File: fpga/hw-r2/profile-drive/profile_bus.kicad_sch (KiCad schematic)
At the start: 13 parts, among them J2 NorComp 182-025-213R561, U1 LFE5U-12F-6TG144C, U2 74LVC245A DATA, U3 74LVC245A CTRL-IN

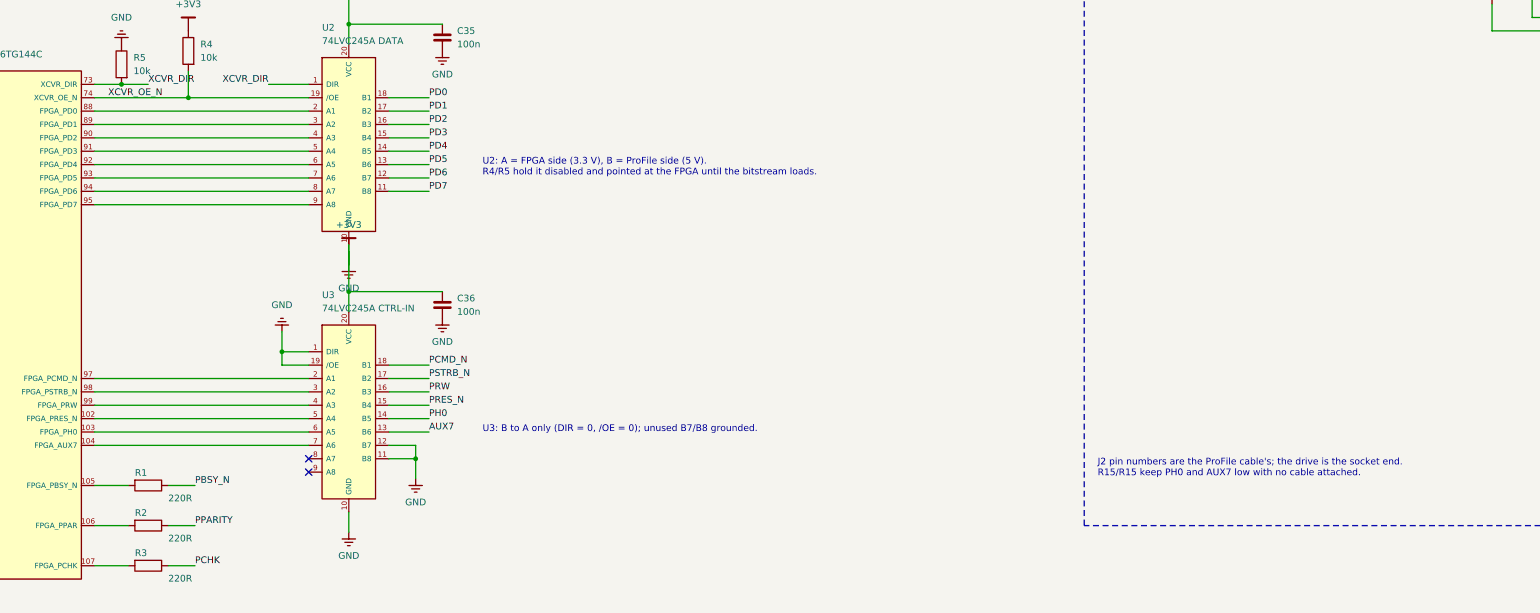
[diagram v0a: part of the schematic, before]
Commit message: more fixes, and r2 gerber first pass
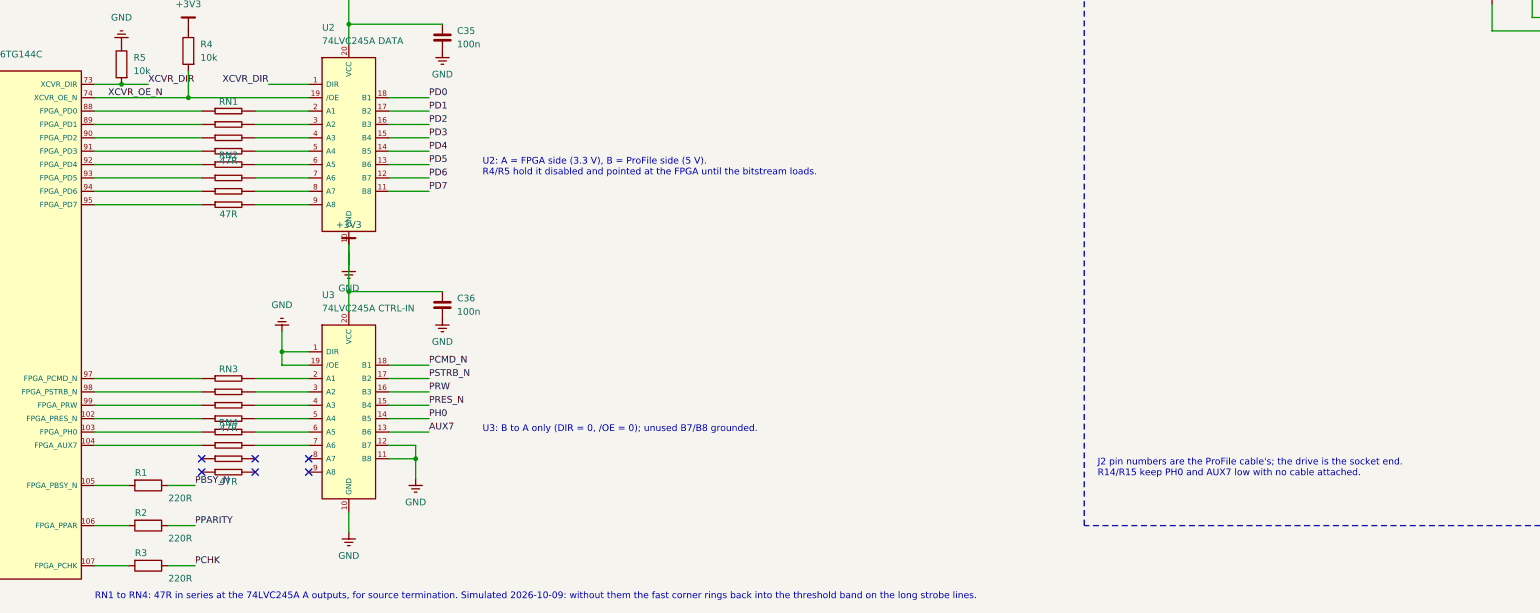
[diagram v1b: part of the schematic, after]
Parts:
- added RN1, RN2, RN3, RN4: 47R, Resistor_SMD:R_Array_Convex_4x0603, symbol device:R_Pack04
- C35, C36: MPN (none) -> Samsung CL10B104KO8NNNC
- J2: MPN (none) -> NorComp 182-025-213R561
- R1, R2, R3: MPN (none) -> Yageo RC0603FR-07220RL
- R14, R15: MPN (none) -> Yageo RC0603FR-07100KL
- R4, R5: MPN (none) -> Yageo RC0603FR-0710KL
- U1: MPN (none) -> Lattice LFE5U-12F-6TG144C
- U2, U3: MPN (none) -> TI SN74LVC245APWR
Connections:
- net at U1.102 (FPGA_PRES_N): now also RN3.4; no longer U3.5 (A4)
- net at U1.103 (FPGA_PH0): now also RN4.1; no longer U3.6 (A5)
- net at U1.104 (FPGA_AUX7): now also RN4.2; no longer U3.7 (A6)
- net at U1.88 (FPGA_PD0): now also RN1.1; no longer U2.2 (A1)
- net at U1.89 (FPGA_PD1): now also RN1.2; no longer U2.3 (A2)
- net at U1.90 (FPGA_PD2): now also RN1.3; no longer U2.4 (A3)
- net at U1.91 (FPGA_PD3): now also RN1.4; no longer U2.5 (A4)
- net at U1.92 (FPGA_PD4): now also RN2.1; no longer U2.6 (A5)
- net at U1.93 (FPGA_PD5): now also RN2.2; no longer U2.7 (A6)
- net at U1.94 (FPGA_PD6): now also RN2.3; no longer U2.8 (A7)
- net at U1.95 (FPGA_PD7): now also RN2.4; no longer U2.9 (A8)
- net at U1.97 (FPGA_PCMD_N): now also RN3.1; no longer U3.2 (A1)
- net at U1.98 (FPGA_PSTRB_N): now also RN3.2; no longer U3.3 (A2)
- net at U1.99 (FPGA_PRW): now also RN3.3; no longer U3.4 (A3)
- new net: RN1.5, U2.5 (A4)
- new net: RN1.6, U2.4 (A3)
- new net: RN1.7, U2.3 (A2)
- new net: RN1.8, U2.2 (A1)
- new net: RN3.8, U3.2 (A1)
- new net: RN3.7, U3.3 (A2)
- new net: RN3.6, U3.4 (A3)
- new net: RN3.5, U3.5 (A4)
- new net: RN4.8, U3.6 (A5)
- new net: RN4.7, U3.7 (A6)
- new net: RN2.8, U2.6 (A5)
- new net: RN2.7, U2.7 (A6)
- new net: RN2.6, U2.8 (A7)
- new net: RN2.5, U2.9 (A8)
- no-connect marks 2 -> 6
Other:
- note added: "J2 pin numbers are the ProFile cable's; the drive is the socket end. R14/R15 keep PH0 and AUX7 low with no cable attached."
- note added: "RN1 to RN4: 47R in series at the 74LVC245A A outputs, for source termination. Simulated 2026-10-09: without them the fast corner rings back into the threshold band on the long strobe lines."
- note removed: "J2 pin numbers are the ProFile cable's; the drive is the socket end. R15/R15 keep PH0 and AUX7 low with no cable attached."
